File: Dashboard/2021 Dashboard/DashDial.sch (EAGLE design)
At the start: 30 parts, among them IC2 TLC5952DAP, J1 ESW-104-23-L-D, J2 ESW-104-23-L-D

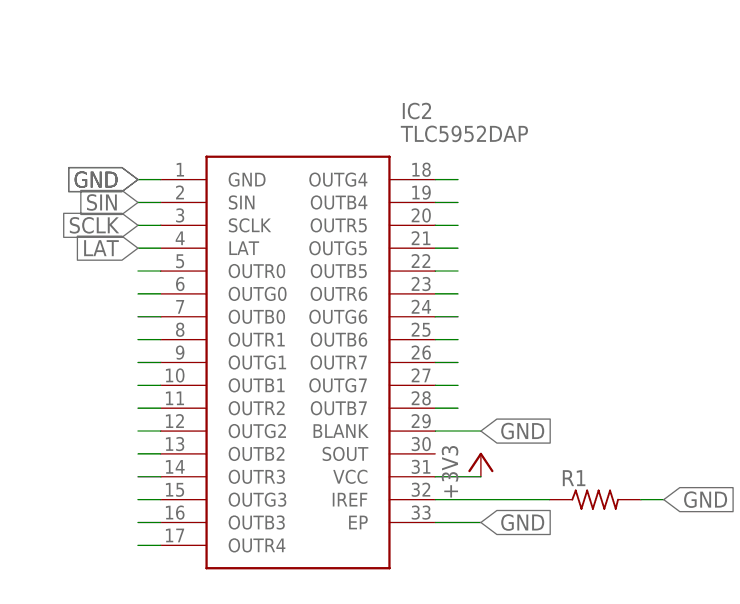
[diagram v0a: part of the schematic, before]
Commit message: Fixed the dashhub #everything
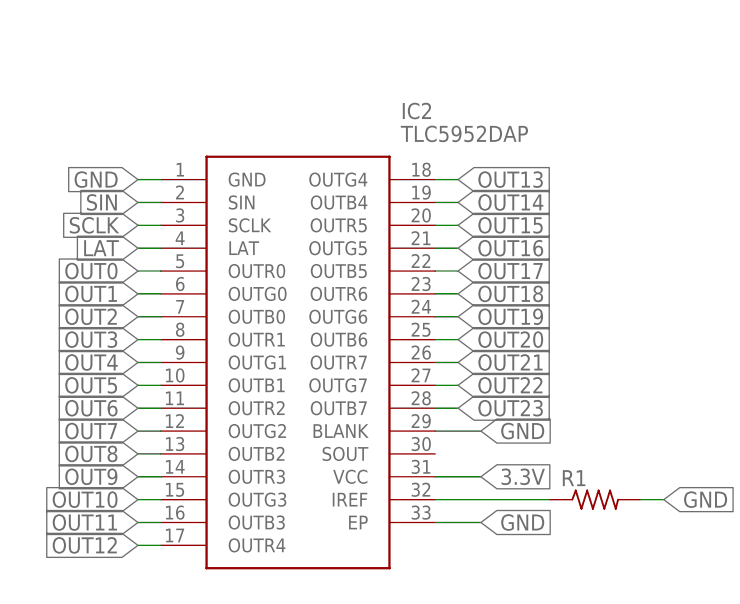
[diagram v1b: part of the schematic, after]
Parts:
- SERVO, SERVO1: device GTOR - Microfit Connector:HEADER_POS3_43650-0315 -> GTOR - Microfit Connector:HEADER_POS3_43650-0300
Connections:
- removed net +3V3: IC2.VCC
- removed net N$30: IC2.GND
- net 3.3V: now also IC2.VCC
- net GND: now also IC2.GND
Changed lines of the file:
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@@
 <part name="J2" library="ESW-104-23-L-D" deviceset="ESW-104-23-L-D" device=""/>
 <part name="IC2" library="GTOR - Active Components" deviceset="TLC5952DAP" device=""/>
-<part name="+3V5" library="GTOR - Documation Frame" deviceset="+3V3" device=""/>
-<part name="SERVO" library="GTOR - Microfit Connector" deviceset="HEADER_POS3_?" device="43650-0315"/>
+<part name="SERVO" library="GTOR - Microfit Connector" deviceset="HEADER_POS3_?" device="43650-0300"/>
 <part name="R1" library="GTOR - Passive Components" deviceset="RES_SMD" device="R0603" package3d_urn="urn:adsk.eagle:package:23555/3"/>
-<part name="SERVO1" library="GTOR - Microfit Connector" deviceset="HEADER_POS3_?" device="43650-0315"/>
+<part name="SERVO1" library="GTOR - Microfit Connector" deviceset="HEADER_POS3_?" device="43650-0300"/>
 </parts>
 <sheets>
@@
 <attribute name="VALUE" x="-3.81" y="78.74" size="1.778" layer="96" align="center-left"/>
 </instance>
-<instance part="+3V5" gate="G$1" x="5.08" y="43.18" smashed="yes">
-<attribute name="VALUE" x="2.54" y="38.1" size="1.778" layer="96" rot="R90"/>
-</instance>
 <instance part="SERVO" gate="G$1" x="45.72" y="111.76" smashed="yes">
 <attribute name="VALUE" x="44.45" y="104.14" size="1.778" layer="96"/>
@@
 <label x="-35.56" y="114.3" size="1.778" layer="95" rot="R180" xref="yes"/>
 </segment>
+<segment>
+<wire x1="0" y1="40.64" x2="5.08" y2="40.64" width="0.1524" layer="91"/>
+<pinref part="IC2" gate="G$1" pin="VCC"/>
+<label x="5.08" y="40.64" size="1.778" layer="95" xref="yes"/>
+</segment>
 </net>
 <net name="GND" class="0">
@@
 </segment>
 <segment>
-<label x="-33.02" y="73.66" size="1.778" layer="95" rot="R180" xref="yes"/>
-<label x="-33.02" y="73.66" size="1.778" layer="95" rot="R180" xref="yes"/>
-</segment>
-<segment>
 <wire x1="22.86" y1="38.1" x2="25.4" y2="38.1" width="0.1524" layer="91"/>
 <label x="25.4" y="38.1" size="1.778" layer="95" xref="yes"/>
@@
 <pinref part="SERVO1" gate="G$1" pin="3"/>
 </segment>
+<segment>
+<pinref part="IC2" gate="G$1" pin="GND"/>
+<wire x1="-30.48" y1="73.66" x2="-33.02" y2="73.66" width="0.1524" layer="91"/>
+<label x="-33.02" y="73.66" size="1.778" layer="95" rot="R180" xref="yes"/>
+</segment>
 </net>
 <net name="7.4V" class="0">
@@
 <pinref part="IC2" gate="G$1" pin="OUTR0"/>
 <wire x1="-33.02" y1="63.5" x2="-30.48" y2="63.5" width="0.1524" layer="91"/>
+<label x="-33.02" y="63.5" size="1.778" layer="95" rot="R180" xref="yes"/>
 </segment>
 </net>
@@
 <pinref part="IC2" gate="G$1" pin="OUTG0"/>
 <wire x1="-30.48" y1="60.96" x2="-33.02" y2="60.96" width="0.1524" layer="91"/>
+<label x="-33.02" y="60.96" size="1.778" layer="95" rot="R180" xref="yes"/>
 </segment>
 </net>
@@
 <pinref part="IC2" gate="G$1" pin="OUTB0"/>
 <wire x1="-30.48" y1="58.42" x2="-33.02" y2="58.42" width="0.1524" layer="91"/>
+<label x="-33.02" y="58.42" size="1.778" layer="95" rot="R180" xref="yes"/>
 </segment>
 </net>
@@
 <pinref part="IC2" gate="G$1" pin="OUTR1"/>
 <wire x1="-33.02" y1="55.88" x2="-30.48" y2="55.88" width="0.1524" layer="91"/>
+<label x="-33.02" y="55.88" size="1.778" layer="95" rot="R180" xref="yes"/>
 </segment>
 </net>
@@
 <pinref part="IC2" gate="G$1" pin="OUTG1"/>
 <wire x1="-33.02" y1="53.34" x2="-30.48" y2="53.34" width="0.1524" layer="91"/>
+<label x="-33.02" y="53.34" size="1.778" layer="95" rot="R180" xref="yes"/>
 </segment>
 </net>
@@
 <pinref part="IC2" gate="G$1" pin="OUTB1"/>
 <wire x1="-30.48" y1="50.8" x2="-33.02" y2="50.8" width="0.1524" layer="91"/>
+<label x="-33.02" y="50.8" size="1.778" layer="95" rot="R180" xref="yes"/>
 </segment>
 </net>
@@
 <pinref part="IC2" gate="G$1" pin="OUTR2"/>
 <wire x1="-33.02" y1="48.26" x2="-30.48" y2="48.26" width="0.1524" layer="91"/>
+<label x="-33.02" y="48.26" size="1.778" layer="95" rot="R180" xref="yes"/>
 </segment>
 </net>
@@
 <pinref part="IC2" gate="G$1" pin="OUTG2"/>
 <wire x1="-33.02" y1="45.72" x2="-30.48" y2="45.72" width="0.1524" layer="91"/>
+<label x="-33.02" y="45.72" size="1.778" layer="95" rot="R180" xref="yes"/>
 </segment>
 </net>
@@
 <pinref part="IC2" gate="G$1" pin="OUTB2"/>
 <wire x1="-33.02" y1="43.18" x2="-30.48" y2="43.18" width="0.1524" layer="91"/>
+<label x="-33.02" y="43.18" size="1.778" layer="95" rot="R180" xref="yes"/>
 </segment>
 </net>
@@
 <pinref part="IC2" gate="G$1" pin="OUTR3"/>
 <wire x1="-30.48" y1="40.64" x2="-33.02" y2="40.64" width="0.1524" layer="91"/>
+<label x="-33.02" y="40.64" size="1.778" layer="95" rot="R180" xref="yes"/>
 </segment>
 </net>
@@
 <pinref part="IC2" gate="G$1" pin="OUTG3"/>
 <wire x1="-33.02" y1="38.1" x2="-30.48" y2="38.1" width="0.1524" layer="91"/>
+<label x="-33.02" y="38.1" size="1.778" layer="95" rot="R180" xref="yes"/>
 </segment>
 </net>
@@
 <pinref part="IC2" gate="G$1" pin="OUTB3"/>
 <wire x1="-33.02" y1="35.56" x2="-30.48" y2="35.56" width="0.1524" layer="91"/>
+<label x="-33.02" y="35.56" size="1.778" layer="95" rot="R180" xref="yes"/>
 </segment>
 </net>
@@
 <pinref part="IC2" gate="G$1" pin="OUTR4"/>
 <wire x1="-33.02" y1="33.02" x2="-30.48" y2="33.02" width="0.1524" layer="91"/>
+<label x="-33.02" y="33.02" size="1.778" layer="95" rot="R180" xref="yes"/>
 </segment>
 </net>
@@
 <pinref part="IC2" gate="G$1" pin="OUTG4"/>
 <wire x1="2.54" y1="73.66" x2="0" y2="73.66" width="0.1524" layer="91"/>
+<label x="2.54" y="73.66" size="1.778" layer="95" xref="yes"/>
 </segment>
 </net>
@@
 <pinref part="IC2" gate="G$1" pin="OUTB4"/>
 <wire x1="0" y1="71.12" x2="2.54" y2="71.12" width="0.1524" layer="91"/>
+<label x="2.54" y="71.12" size="1.778" layer="95" xref="yes"/>
 </segment>
 </net>
@@
 <pinref part="IC2" gate="G$1" pin="OUTR5"/>
 <wire x1="2.54" y1="68.58" x2="0" y2="68.58" width="0.1524" layer="91"/>
+<label x="2.54" y="68.58" size="1.778" layer="95" xref="yes"/>
 </segment>
 </net>
@@
 <pinref part="IC2" gate="G$1" pin="OUTG5"/>
 <wire x1="2.54" y1="66.04" x2="0" y2="66.04" width="0.1524" layer="91"/>
+<label x="2.54" y="66.04" size="1.778" layer="95" xref="yes"/>
 </segment>
 </net>
@@
 <pinref part="IC2" gate="G$1" pin="OUTB5"/>
 <wire x1="2.54" y1="63.5" x2="0" y2="63.5" width="0.1524" layer="91"/>
+<label x="2.54" y="63.5" size="1.778" layer="95" xref="yes"/>
 </segment>
 </net>
@@
 <pinref part="IC2" gate="G$1" pin="OUTR6"/>
 <wire x1="0" y1="60.96" x2="2.54" y2="60.96" width="0.1524" layer="91"/>
+<label x="2.54" y="60.96" size="1.778" layer="95" xref="yes"/>
 </segment>
 </net>
@@
 <pinref part="IC2" gate="G$1" pin="OUTG6"/>
 <wire x1="2.54" y1="58.42" x2="0" y2="58.42" width="0.1524" layer="91"/>
+<label x="2.54" y="58.42" size="1.778" layer="95" xref="yes"/>
 </segment>
 </net>
@@
 <pinref part="IC2" gate="G$1" pin="OUTB6"/>
 <wire x1="2.54" y1="55.88" x2="0" y2="55.88" width="0.1524" layer="91"/>
+<label x="2.54" y="55.88" size="1.778" layer="95" xref="yes"/>
 </segment>
 </net>
@@
 <pinref part="IC2" gate="G$1" pin="OUTR7"/>
 <wire x1="0" y1="53.34" x2="2.54" y2="53.34" width="0.1524" layer="91"/>
+<label x="2.54" y="53.34" size="1.778" layer="95" xref="yes"/>
 </segment>
 </net>
@@
 <pinref part="IC2" gate="G$1" pin="OUTG7"/>
 <wire x1="2.54" y1="50.8" x2="0" y2="50.8" width="0.1524" layer="91"/>
+<label x="2.54" y="50.8" size="1.778" layer="95" xref="yes"/>
 </segment>
 </net>
@@
 <pinref part="IC2" gate="G$1" pin="OUTB7"/>
 <wire x1="2.54" y1="48.26" x2="0" y2="48.26" width="0.1524" layer="91"/>
+<label x="2.54" y="48.26" size="1.778" layer="95" xref="yes"/>
 </segment>
 </net>
@@
 </segment>
 </net>
-<net name="+3V3" class="0">
-<segment>
-<wire x1="0" y1="40.64" x2="5.08" y2="40.64" width="0.1524" layer="91"/>
-<pinref part="IC2" gate="G$1" pin="VCC"/>
-<pinref part="+3V5" gate="G$1" pin="+3V3"/>
-</segment>
-</net>
-<net name="N$30" class="0">
-<segment>
-<wire x1="-30.48" y1="73.66" x2="-33.02" y2="73.66" width="0.1524" layer="91"/>
-<pinref part="IC2" gate="G$1" pin="GND"/>
-</segment>
-</net>
